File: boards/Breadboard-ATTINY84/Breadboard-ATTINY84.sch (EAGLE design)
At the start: 8 parts, among them J1 PINHD-1X7, J2 PINHD-1X7, U1 ATTINY84-20PU

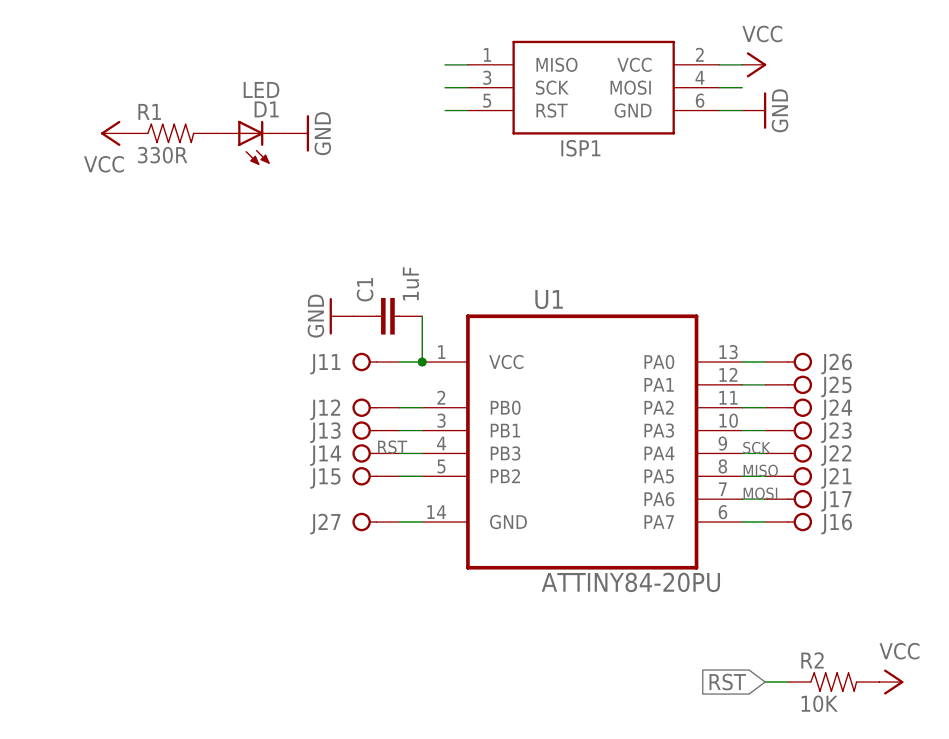
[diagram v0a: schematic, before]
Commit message: Updated breadboard ATTiny84
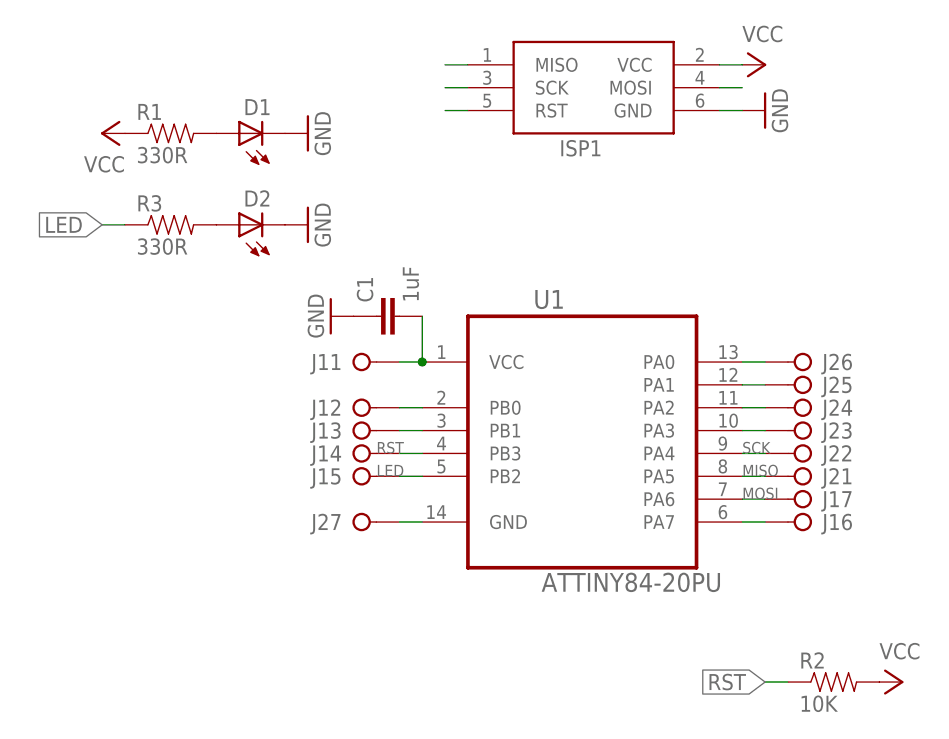
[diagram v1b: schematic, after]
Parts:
- added D2: LED-0805, SaintGimp:LED-0805
- added R3: 330R, SaintGimp:RESISTOR-0805
- D1: value LED -> LED-0805; device SaintGimp:LED -> SaintGimp:LED-0805
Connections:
- removed net N$5: J15.KL, U1.PB2
- new net LED: J15.KL, R3.1, U1.PB2
- new net N$1: D2.A, R3.2
- net GND: now also D2.C
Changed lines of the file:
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@@
 <layer number="112" name="tSilk" color="7" fill="1" visible="yes" active="yes"/>
 <layer number="113" name="IDFDebug" color="7" fill="1" visible="yes" active="yes"/>
+<layer number="114" name="FRNTMAAT1" color="7" fill="1" visible="yes" active="yes"/>
+<layer number="115" name="FRNTMAAT2" color="7" fill="1" visible="yes" active="yes"/>
 <layer number="116" name="Patch_BOT" color="9" fill="4" visible="yes" active="yes"/>
+<layer number="117" name="BACKMAAT1" color="7" fill="1" visible="yes" active="yes"/>
 <layer number="118" name="Rect_Pads" color="7" fill="1" visible="no" active="no"/>
+<layer number="119" name="KAP_TEKEN" color="7" fill="1" visible="yes" active="yes"/>
+<layer number="120" name="KAP_MAAT1" color="7" fill="1" visible="yes" active="yes"/>
 <layer number="121" name="_tsilk" color="7" fill="1" visible="yes" active="yes"/>
 <layer number="122" name="_bsilk" color="7" fill="1" visible="yes" active="yes"/>
@@
 <layer number="128" name="_bValues" color="7" fill="1" visible="yes" active="yes"/>
 <layer number="129" name="Mask" color="7" fill="1" visible="yes" active="yes"/>
+<layer number="130" name="SMDSTROOK" color="7" fill="1" visible="yes" active="yes"/>
 <layer number="131" name="tAdjust" color="7" fill="1" visible="no" active="yes"/>
 <layer number="132" name="bAdjust" color="7" fill="1" visible="no" active="yes"/>
@@
 <part name="C1" library="SaintGimp" deviceset="CAPACITOR-*" device="0805" value="1uF"/>
 <part name="GND2" library="SaintGimp" deviceset="GND" device=""/>
-<part name="D1" library="SaintGimp" deviceset="LED" device=""/>
+<part name="D1" library="SaintGimp" deviceset="LED-*" device="0805"/>
 <part name="GND3" library="SaintGimp" deviceset="GND" device=""/>
 <part name="P+1" library="SaintGimp" deviceset="VCC" device=""/>
@@
 <part name="J1" library="SaintGimp" deviceset="PINHD-1X7" device=""/>
 <part name="J2" library="SaintGimp" deviceset="PINHD-1X7" device=""/>
+<part name="R3" library="SaintGimp" deviceset="RESISTOR-*" device="0805" value="330R"/>
+<part name="D2" library="SaintGimp" deviceset="LED-*" device="0805"/>
+<part name="GND4" library="SaintGimp" deviceset="GND" device=""/>
 </parts>
 <sheets>
@@
 <instance part="J2" gate="6" x="93.98" y="53.34" rot="R180"/>
 <instance part="J2" gate="7" x="43.18" y="35.56"/>
+<instance part="R3" gate="G$1" x="22.86" y="68.58"/>
+<instance part="D2" gate="1" x="33.02" y="68.58" rot="R90"/>
+<instance part="GND4" gate="1" x="38.1" y="68.58" rot="R90"/>
 </instances>
 <busses>
@@
 <wire x1="48.26" y1="35.56" x2="50.8" y2="35.56" width="0.1524" layer="91"/>
 </segment>
+<segment>
+<pinref part="D2" gate="1" pin="C"/>
+<pinref part="GND4" gate="1" pin="GND"/>
+</segment>
 </net>
 <net name="MISO" class="0">
@@
 <pinref part="J1" gate="4" pin="KL"/>
 <wire x1="48.26" y1="43.18" x2="50.8" y2="43.18" width="0.1524" layer="91"/>
-<label x="45.72" y="43.18" size="1.4224" layer="95"/>
+<label x="45.72" y="43.18" size="1.27" layer="95"/>
 </segment>
 <segment>
@@
 </segment>
 </net>
-<net name="N$5" class="0">
+<net name="LED" class="0">
 <segment>
 <pinref part="U1" gate="A" pin="PB2"/>
 <pinref part="J1" gate="5" pin="KL"/>
 <wire x1="48.26" y1="40.64" x2="50.8" y2="40.64" width="0.1524" layer="91"/>
+<label x="45.72" y="40.64" size="1.27" layer="95"/>
+</segment>
+<segment>
+<pinref part="R3" gate="G$1" pin="1"/>
+<wire x1="17.78" y1="68.58" x2="15.24" y2="68.58" width="0.1524" layer="91"/>
+<label x="15.24" y="68.58" size="1.778" layer="95" rot="R180" xref="yes"/>
 </segment>
 </net>
@@
 </segment>
 </net>
+<net name="N$1" class="0">
+<segment>
+<pinref part="D2" gate="1" pin="A"/>
+<pinref part="R3" gate="G$1" pin="2"/>
+</segment>
+</net>
